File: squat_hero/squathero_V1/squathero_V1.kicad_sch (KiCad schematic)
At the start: 6 parts, among them U2 AMS1117

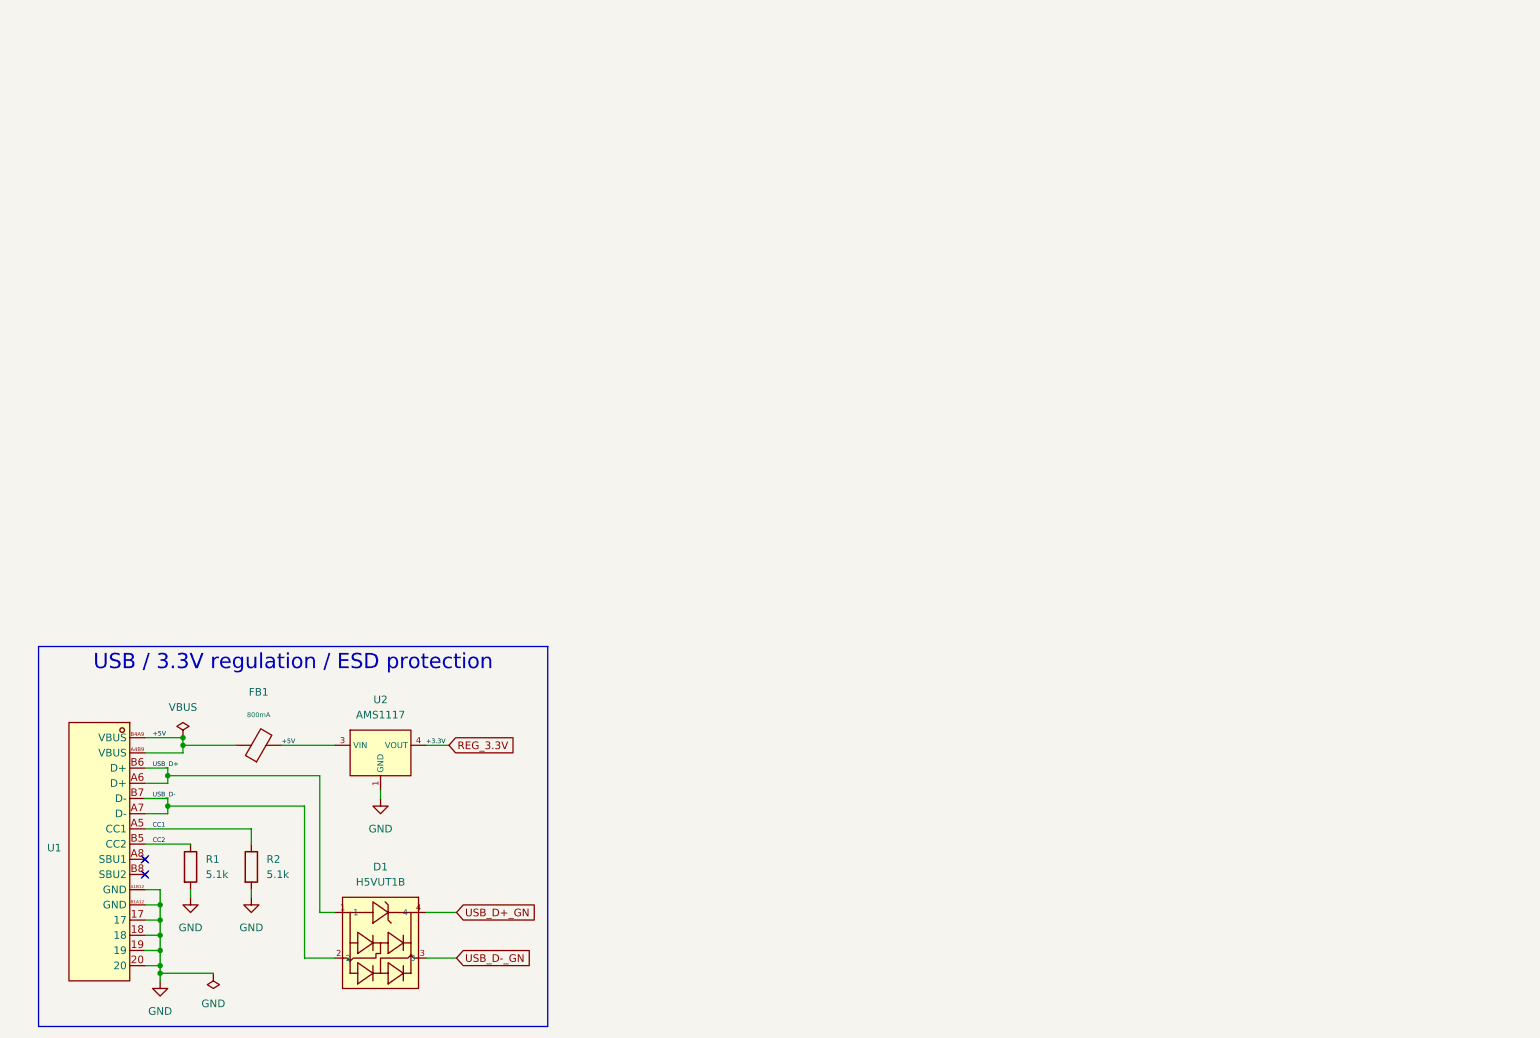
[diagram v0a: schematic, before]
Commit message: V1 squat hero
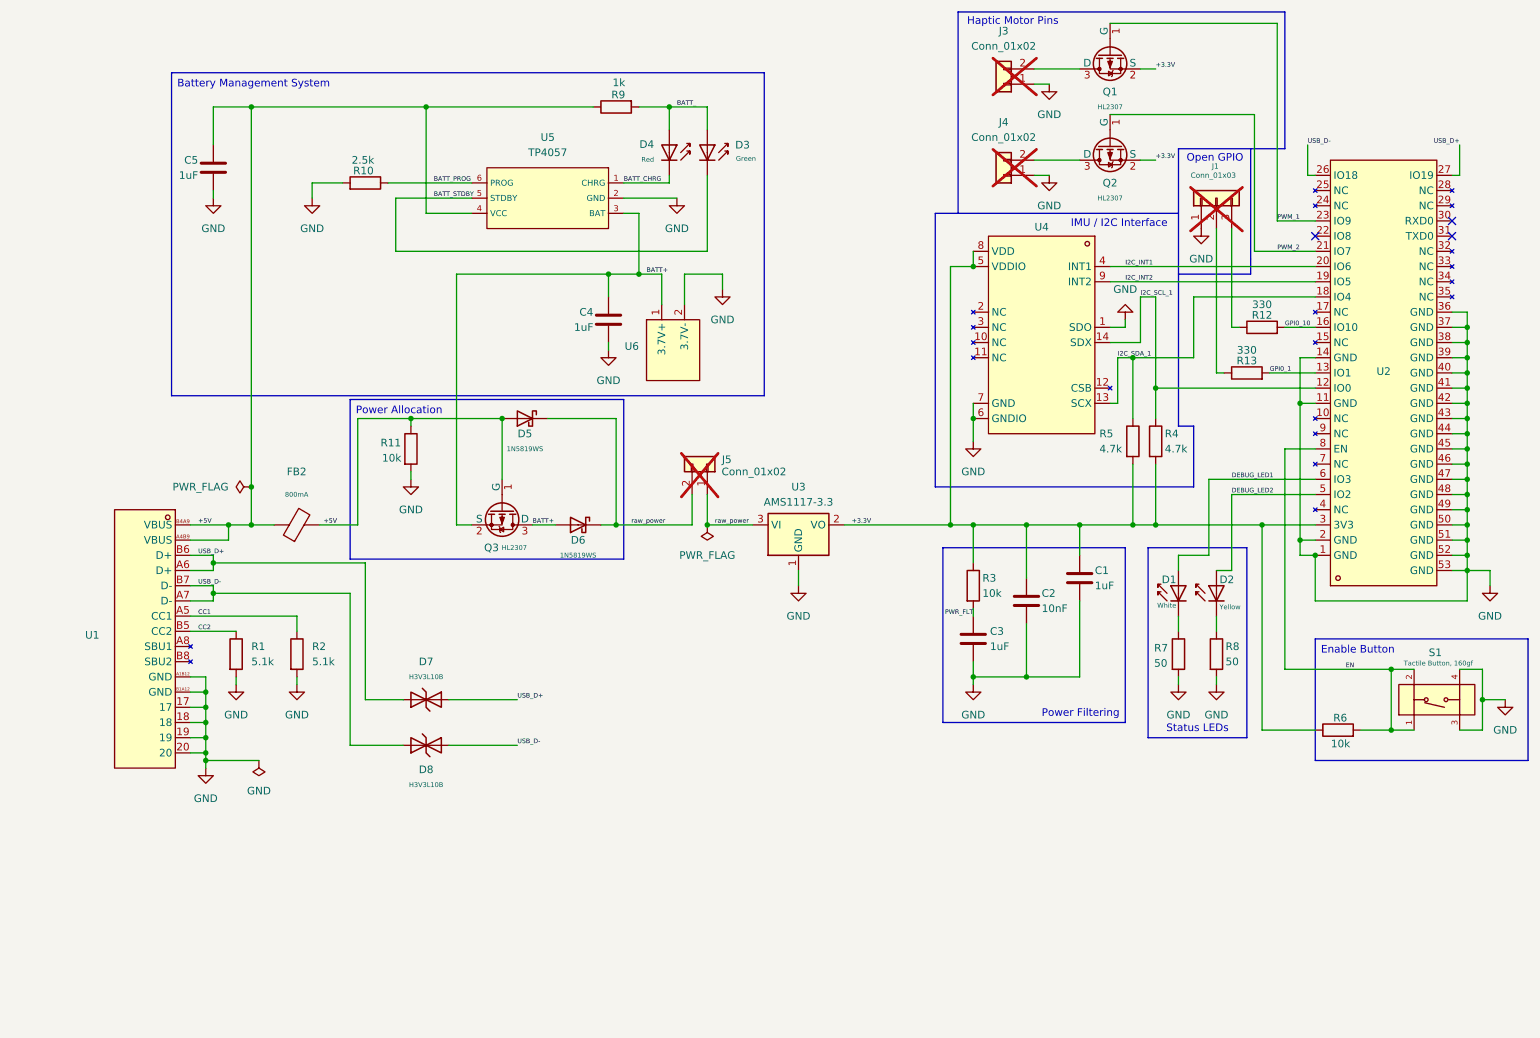
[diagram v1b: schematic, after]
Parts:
- removed D1: H5VUT1B, PCM_JLCPCB:SOT-143-4_L2.9-W1.3-P1.90-LS2.4-BL-1, symbol PCM_JLCPCB-Diode-Packages:Package, H5VUT1B
- removed FB1: ~, PCM_JLCPCB:FB_0805, symbol PCM_JLCPCB-Inductors:Ferrite,0805
- removed U1: ~, JLCPCB_USB-C:USB-SMD_TYPE-C16PIN-1, symbol JLCPCB_USB-C:12402012E212A
- removed U2: AMS1117, PCM_JLCPCB:SOT-223-3_L6.5-W3.4-P2.30-LS7.0-BR, symbol PCM_JLCPCB-Power:LDO, 3.3V, 1A
- added C1, C3, C4, C5: 1uF, Resistor_SMD:R_0805_2012Metric, symbol Device:C
- added C2: 10nF, Resistor_SMD:R_0805_2012Metric, symbol Device:C
- added D1: White, PCM_JLCPCB:D_0805, symbol PCM_JLCPCB-Diodes:LED,0805,White
- added D2: Yellow, PCM_JLCPCB:D_0805, symbol PCM_JLCPCB-Diodes:LED,0805,Yellow
- added D3: Green, PCM_JLCPCB:D_0805, symbol PCM_JLCPCB-Diodes:LED,0805,Green
- added D4: Red, PCM_JLCPCB:D_0603, symbol PCM_JLCPCB-Diodes:LED,0603,Red
- added D5, D6: 1N5819WS, PCM_JLCPCB:D_SOD-323, symbol PCM_JLCPCB-Diodes:Schottky,1N5819WS
- added D7, D8: H3V3L10B, PCM_JLCPCB:D_DFN1006-2L, symbol PCM_JLCPCB-Diodes:TVS-Bi,H3V3L10B
- added FB2: ~, PCM_JLCPCB:FB_0805, symbol PCM_JLCPCB-Inductors:Ferrite,0805
- added J1: Conn_01x03, Connector_PinSocket_2.54mm:PinSocket_1x03_P2.54mm_Vertical, symbol Connector_Generic:Conn_01x03
- added J3, J4, J5: Conn_01x02, Connector_PinSocket_2.54mm:PinSocket_1x02_P2.54mm_Vertical, symbol Connector_Generic:Conn_01x02
- added Q1, Q2, Q3: HL2307, PCM_JLCPCB:Q_SOT-23, symbol PCM_JLCPCB-Transistors:PMOS,HL2307
- added R10: 2.5k, Resistor_SMD:R_0805_2012Metric, symbol Device:R
- added R11, R3, R6: 10k, Resistor_SMD:R_0805_2012Metric, symbol Device:R
- added R12, R13: 330, Resistor_SMD:R_0805_2012Metric, symbol Device:R
- added R4, R5: 4.7k, Resistor_SMD:R_0805_2012Metric, symbol Device:R
- added R7, R8: 50, Resistor_SMD:R_0805_2012Metric, symbol Device:R
- added R9: 1k, Resistor_SMD:R_0805_2012Metric, symbol Device:R
- added S1: Tactile Button, 160gf, PCM_JLCPCB:SW-SMD_4P-L5.1-W5.1-P3.70-LS6.5-TL-2, symbol PCM_JLCPCB-Connectors_Buttons:Tactile Button, 160gf
- added U1: ~, JLCPCB_USB_FOOTPRINT:USB-SMD_TYPE-C16PIN-1, symbol JLCPCB_USBC:12402012E212A
- added U2: ~, esp_32:WIFIM-SMD_ESP32-C3-MINI-1, symbol esp_32:ESP32-C3-MINI-1-N4
- added U3: AMS1117-3.3, Package_TO_SOT_SMD:SOT-223-3_TabPin2, symbol Regulator_Linear:AMS1117-3.3
- added U4: ~, imu:LGA-14_L3.0-W2.5-P0.50-TL_QMI8658A, symbol imu:BMI323
- added U5: TP4057, PCM_JLCPCB:SOT-23-6_L2.9-W1.6-P0.95-LS2.8-BL, symbol PCM_JLCPCB-Power:Battery, Li-Ion, 0.5A, TP4057
- added U6: ~, batt_conn:Untitled, symbol batt_conn:3.7V_batt_pads
- R1, R2: footprint Resistor_SMD:R_0805_2012Metric -> Resistor_SMD:R_0201_0603Metric
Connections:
- net +5V: now also C5.1, D5.2, FB2.1, FB2.2, Q3.1 (G), R11.1, R9.1, U1.A4B9 (VBUS), U1.B4A9 (VBUS), U5.4 (VCC)
- net CC1: now also U1.A5 (CC1)
- net CC2: now also U1.B5 (CC2)
- net GND: now also C1.2, C2.2, C3.2, C4.2, C5.2, J1.1 (Pin_1), J3.1 (Pin_1), J4.1 (Pin_1), R10.2, R11.2, R7.2, R8.2, S1.3 (C), S1.4 (D), U1.17, U1.18, U1.19, U1.20, U1.A1B12 (GND), U1.B1A12 (GND), U2.1 (GND), U2.11 (GND), U2.14 (GND), U2.2 (GND), U2.36 (GND), U2.37 (GND), U2.38 (GND), U2.39 (GND), U2.40 (GND), U2.41 (GND), U2.42 (GND), U2.43 (GND), U2.44 (GND), U2.45 (GND), U2.46 (GND), U2.47 (GND), U2.48 (GND), U2.49 (GND), U2.50 (GND), U2.51 (GND), U2.52 (GND), U2.53 (GND), U3.1 (GND), U4.1 (SDO), U4.6 (GNDIO), U4.7 (GND), U5.2 (GND), U6.2 (3.7V-)
- net USB_D+: now also D7.1, D7.2, U1.A6 (D+), U1.B6 (D+), U2.27 (IO19)
- net USB_D-: now also D8.1, D8.2, U1.A7 (D-), U1.B7 (D-), U2.26 (IO18)
- new net: J3.2 (Pin_2), Q1.3 (D)
- new net: J1.3 (Pin_3), R12.1
- new net: D1.1, R7.1
- new net: J4.2 (Pin_2), Q2.3 (D)
- new net: J1.2 (Pin_2), R13.1
- new net: D2.1, R8.1
- new net +3.3V: C1.1, C2.1, Q1.2 (S), Q2.2 (S), R3.1, R4.2, R5.2, R6.1, U2.3 (3V3), U3.2 (VO), U4.5 (VDDIO), U4.8 (VDD)
- new net BATT+: C4.1, D6.2, Q3.2 (S), Q3.3 (D), U5.3 (BAT), U6.1 (3.7V+)
- new net BATT_: D3.2, D4.2, R9.2
- new net BATT_CHRG: D4.1, U5.1 (CHRG)
- new net BATT_PROG: R10.1, U5.6 (PROG)
- new net BATT_STDBY: D3.1, U5.5 (STDBY)
- new net DEBUG_LED1: D1.2, U2.6 (IO3)
- new net DEBUG_LED2: D2.2, U2.5 (IO2)
- new net EN: R6.2, S1.1 (A), S1.2 (B), U2.8 (EN)
- new net GPI0_1: R13.2, U2.13 (IO1)
- new net GPI0_10: R12.2, U2.16 (IO10)
- new net I2C_INT1: U2.20 (IO6), U4.4 (INT1)
- new net I2C_INT2: U2.19 (IO5), U4.9 (INT2)
- new net I2C_SCL_1: R4.1, U2.12 (IO0), U4.14 (SDX)
- new net I2C_SDA_1: R5.1, U2.18 (IO4), U4.13 (SCX)
- new net PWM_1: Q1.1 (G), U2.23 (IO9)
- new net PWM_2: Q2.1 (G), U2.21 (IO7)
- new net PWR_FLT: C3.1, R3.2
- new net raw_power: D5.1, D6.1, J5.1 (Pin_1), J5.2 (Pin_2), U3.3 (VI)
- no-connect marks 2 -> 3
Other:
- note added: "Haptic Motor Pins"
- note added: "IMU / I2C Interface"
- note added: "Open GPIO"
- moved on the sheet: R1, R2
